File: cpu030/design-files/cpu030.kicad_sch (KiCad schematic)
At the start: 65 parts, among them J101 Reset, J102 SYSCTL JTAG, J103 NMI, SW101 Reset, SW102 NMI, U101 MC68030RC, U102 ATF1508AS, U103 MC74ACT05DG, U104 DS1813, U105 SST39SF040 (E), U106 SST39SF040 (O), U107 MC68882, U108 GAL22V10, U109 MC74ACT05DG, U110 DS1813, Y101 50MHz

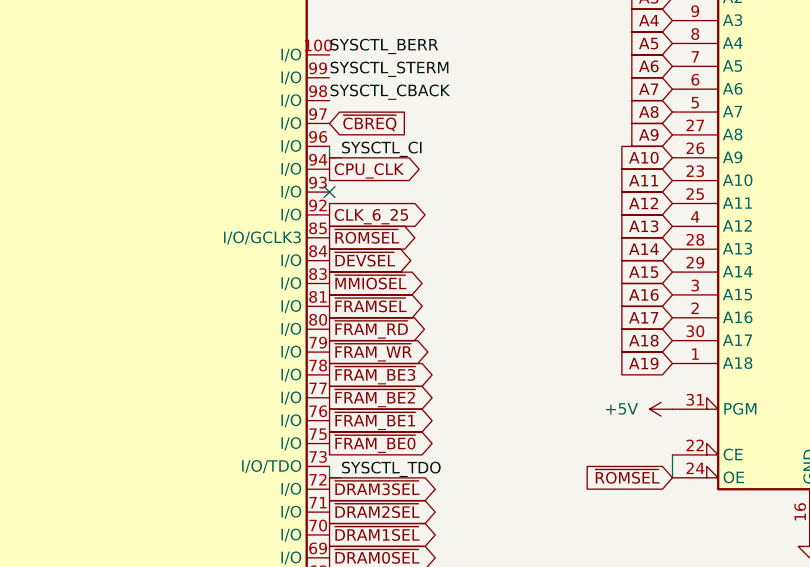
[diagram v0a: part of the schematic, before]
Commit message: MMIOSEL -> EXPSEL
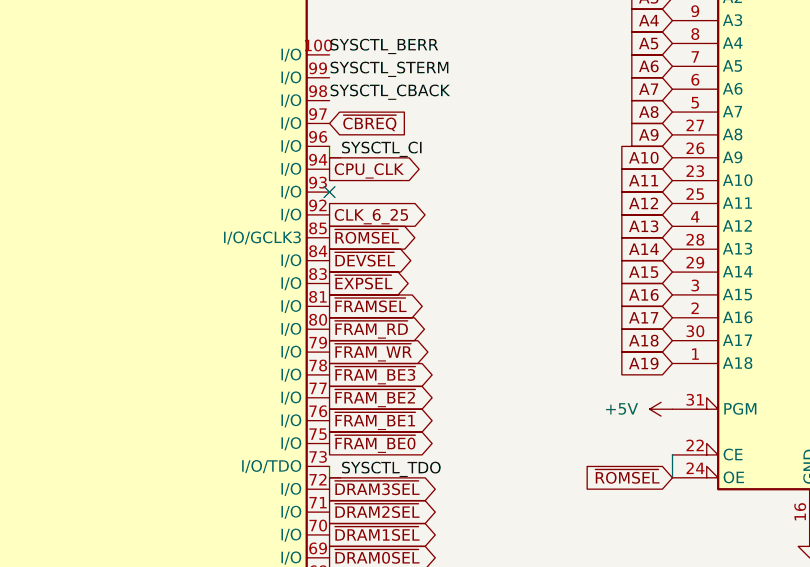
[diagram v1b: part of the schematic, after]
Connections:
- net ~{MMIOSEL} renamed ~{EXPSEL}
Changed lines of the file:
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@@
 		)
 	)
-	(global_label "~{MMIOSEL}"
+	(global_label "~{EXPSEL}"
 		(shape output)
 		(at 264.16 63.5 0)
@@
 		)
 		(property "Intersheetrefs" "${INTERSHEET_REFS}"
-			(at 275.3699 63.5 0)
+			(at 274.1603 63.5 0)
 			(effects
 				(font
